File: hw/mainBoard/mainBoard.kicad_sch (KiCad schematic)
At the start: 0 parts

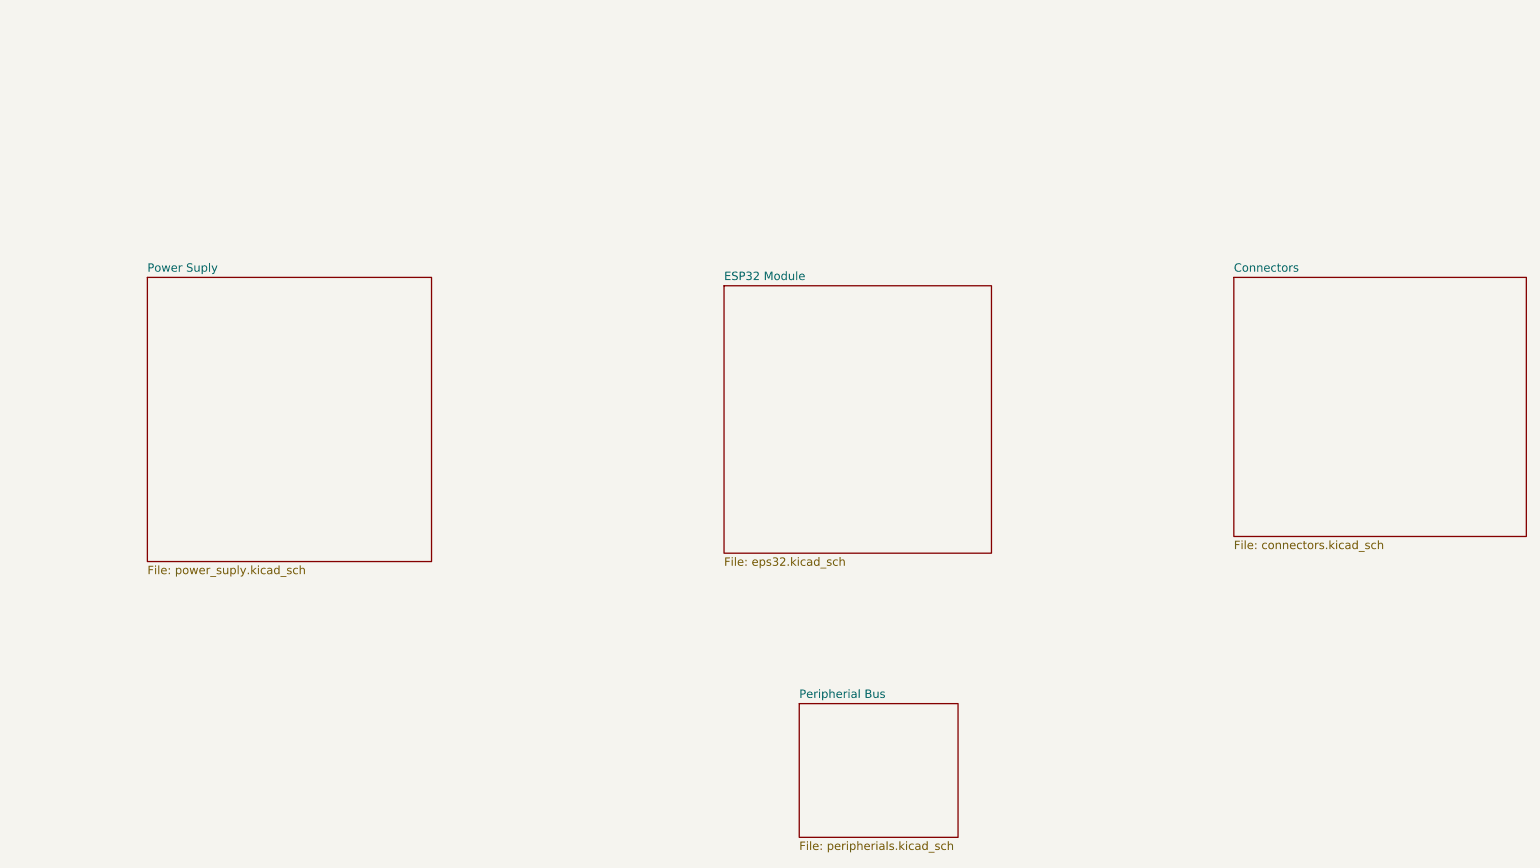
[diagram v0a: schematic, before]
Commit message: hw + blok schema
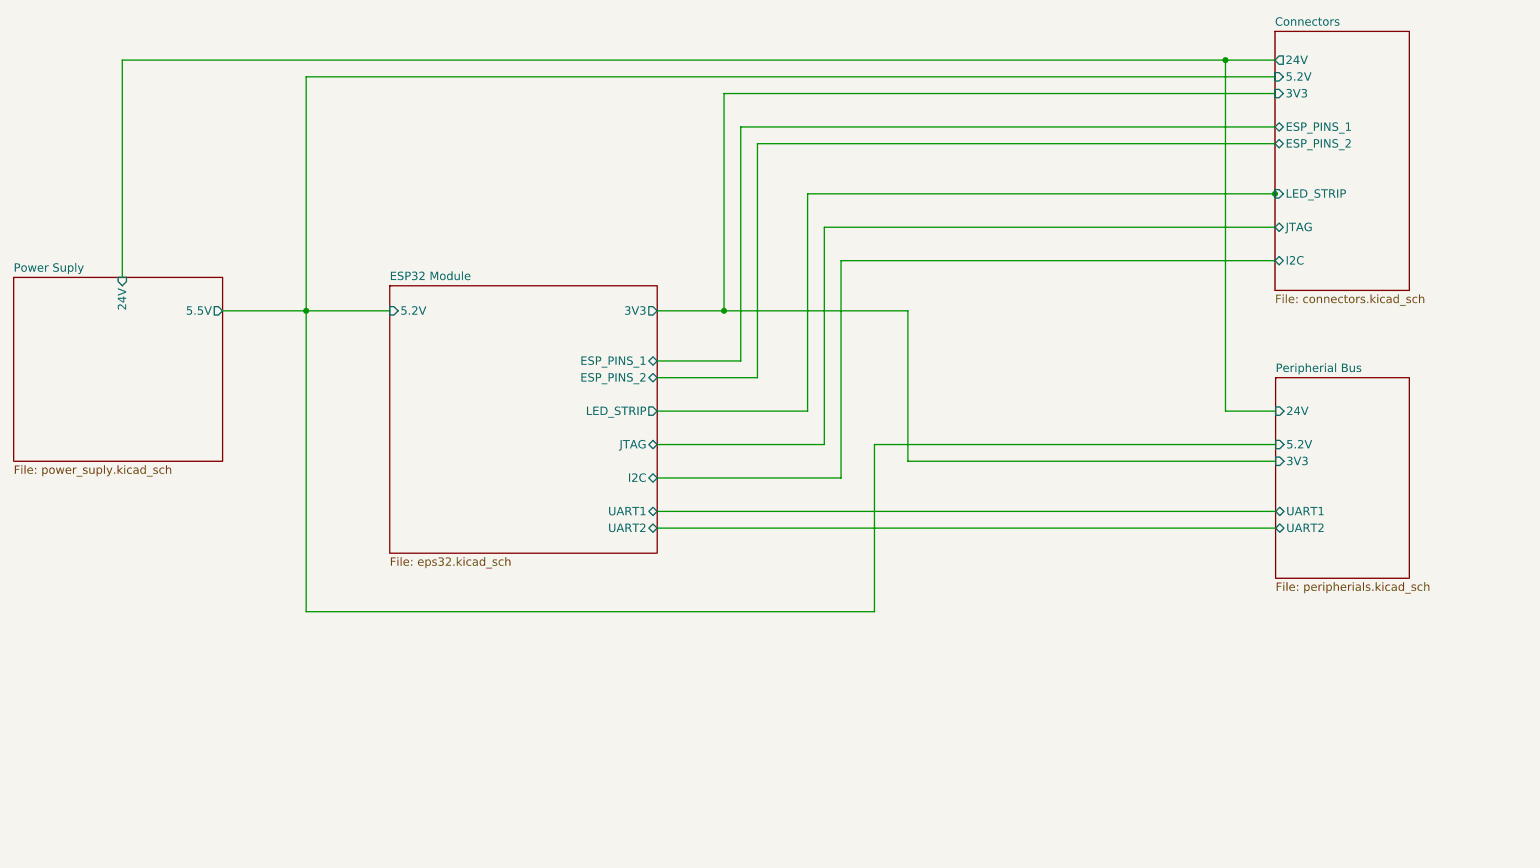
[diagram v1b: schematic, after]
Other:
- sheet Connectors ports: added 24V, 3V3, 5.2V, ESP_PINS_1, ESP_PINS_2, I2C, JTAG, LED_STRIP; removed none
- sheet ESP32 Module ports: added 3V3, 5.2V, ESP_PINS_1, ESP_PINS_2, I2C, JTAG, LED_STRIP, UART1, UART2; removed none
- sheet Peripherial Bus ports: added 24V, 3V3, 5.2V, UART1, UART2; removed none
- sheet Power Suply ports: added 24V, 5.5V; removed none
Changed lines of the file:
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@@
 (kicad_sch (version 20230121) (generator eeschema)
   (paper "A4")
-  (sheet (at 151.13 133.35) (size 24.13 20.32) (fields_autoplaced)
-    (stroke (width 0.1524) (type solid))
-    (fill (color 0 0 0 0.0000))
-    (property "Sheetname" "Peripherial Bus" (at 151.13 132.6384 0)
-      (effects (font (size 1.27 1.27)) (justify left bottom))
-    )
-    (property "Sheetfile" "peripherials.kicad_sch" (at 151.13 154.2546 0)
-      (effects (font (size 1.27 1.27)) (justify left top))
+  (junction (at 215.9 35.56) (diameter 0) (color 0 0 0 0)
+  )
+  (junction (at 139.7 73.66) (diameter 0) (color 0 0 0 0)
+  )
+  (junction (at 223.4202 55.88) (diameter 0) (color 0 0 0 0)
+  )
+  (junction (at 76.2 73.66) (diameter 0) (color 0 0 0 0)
+  )
+  (wire (pts (xy 76.2 119.38) (xy 162.56 119.38))
+    (stroke (width 0) (type default))
+  )
+  (wire (pts (xy 76.2 73.66) (xy 76.2 38.1))
+    (stroke (width 0) (type default))
+  )
+  (wire (pts (xy 152.4 55.88) (xy 223.4202 55.88))
+    (stroke (width 0) (type default))
+  )
+  (wire (pts (xy 129.54 81.28) (xy 142.24 81.28))
+    (stroke (width 0) (type default))
+  )
+  (wire (pts (xy 162.56 93.98) (xy 223.52 93.98))
+    (stroke (width 0) (type default))
+  )
+  (wire (pts (xy 63.5 73.66) (xy 76.2 73.66))
+    (stroke (width 0) (type default))
+  )
+  (wire (pts (xy 139.7 40.64) (xy 223.4202 40.64))
+    (stroke (width 0) (type default))
+  )
+  (wire (pts (xy 76.2 38.1) (xy 223.4202 38.1))
+    (stroke (width 0) (type default))
+  )
+  (wire (pts (xy 129.54 88.9) (xy 152.4 88.9))
+    (stroke (width 0) (type default))
+  )
+  (wire (pts (xy 48.26 35.56) (xy 48.26 68.58))
+    (stroke (width 0) (type default))
+  )
+  (wire (pts (xy 129.54 104.14) (xy 223.52 104.14))
+    (stroke (width 0) (type default))
+  )
+  (wire (pts (xy 167.64 96.52) (xy 223.52 96.52))
+    (stroke (width 0) (type default))
+  )
+  (wire (pts (xy 142.24 45.72) (xy 223.4202 45.72))
+    (stroke (width 0) (type default))
+  )
+  (wire (pts (xy 139.7 73.66) (xy 139.7 40.64))
+    (stroke (width 0) (type default))
+  )
+  (wire (pts (xy 129.54 83.82) (xy 144.78 83.82))
+    (stroke (width 0) (type default))
+  )
+  (wire (pts (xy 162.56 119.38) (xy 162.56 93.98))
+    (stroke (width 0) (type default))
+  )
+  (wire (pts (xy 152.4 88.9) (xy 152.4 55.88))
+    (stroke (width 0) (type default))
+  )
+  (wire (pts (xy 76.2 73.66) (xy 76.2 119.38))
+    (stroke (width 0) (type default))
+  )
+  (wire (pts (xy 157.48 99.06) (xy 157.48 66.04))
+    (stroke (width 0) (type default))
+  )
+  (wire (pts (xy 223.4202 55.88) (xy 223.52 55.88))
+    (stroke (width 0) (type default))
+  )
+  (wire (pts (xy 129.54 99.06) (xy 157.48 99.06))
+    (stroke (width 0) (type default))
+  )
+  (wire (pts (xy 129.54 93.98) (xy 154.94 93.98))
+    (stroke (width 0) (type default))
+  )
+  (wire (pts (xy 142.24 81.28) (xy 142.24 45.72))
+    (stroke (width 0) (type default))
+  )
+  (wire (pts (xy 129.54 73.66) (xy 139.7 73.66))
+    (stroke (width 0) (type default))
+  )
+  (wire (pts (xy 157.48 66.04) (xy 223.4202 66.04))
+    (stroke (width 0) (type default))
+  )
+  (wire (pts (xy 144.78 48.26) (xy 223.4202 48.26))
+    (stroke (width 0) (type default))
+  )
+  (wire (pts (xy 76.2 73.66) (xy 88.9 73.66))
+    (stroke (width 0) (type default))
+  )
+  (wire (pts (xy 215.9 35.56) (xy 48.26 35.56))
+    (stroke (width 0) (type default))
+  )
+  (wire (pts (xy 167.64 73.66) (xy 167.64 96.52))
+    (stroke (width 0) (type default))
+  )
+  (wire (pts (xy 139.7 73.66) (xy 167.64 73.66))
+    (stroke (width 0) (type default))
+  )
+  (wire (pts (xy 223.52 88.9) (xy 215.9 88.9))
+    (stroke (width 0) (type default))
+  )
+  (wire (pts (xy 144.78 83.82) (xy 144.78 48.26))
+    (stroke (width 0) (type default))
+  )
+  (wire (pts (xy 215.9 35.56) (xy 215.9 88.9))
+    (stroke (width 0) (type default))
+  )
+  (wire (pts (xy 154.94 60.96) (xy 223.4202 60.96))
+    (stroke (width 0) (type default))
+  )
+  (wire (pts (xy 129.54 106.68) (xy 223.52 106.68))
+    (stroke (width 0) (type default))
+  )
+  (wire (pts (xy 223.4202 35.56) (xy 215.9 35.56))
+    (stroke (width 0) (type default))
+  )
+  (wire (pts (xy 154.94 93.98) (xy 154.94 60.96))
+    (stroke (width 0) (type default))
+  )
+  (sheet (at 223.52 83.82) (size 20.32 30.48) (fields_autoplaced)
+    (stroke (width 0.1524) (type solid))
+    (fill (color 0 0 0 0.0000))
+    (property "Sheetname" "Peripherial Bus" (at 223.52 83.1084 0)
+      (effects (font (size 1.27 1.27)) (justify left bottom))
+    )
+    (property "Sheetfile" "peripherials.kicad_sch" (at 223.52 114.8846 0)
+      (effects (font (size 1.27 1.27)) (justify left top))
+    )
+    (pin "UART2" bidirectional (at 223.52 106.68 180)
+      (effects (font (size 1.27 1.27)) (justify left))
+    )
+    (pin "UART1" bidirectional (at 223.52 104.14 180)
+      (effects (font (size 1.27 1.27)) (justify left))
+    )
+    (pin "3V3" input (at 223.52 96.52 180)
+      (effects (font (size 1.27 1.27)) (justify left))
+    )
+    (pin "5.2V" input (at 223.52 93.98 180)
+      (effects (font (size 1.27 1.27)) (justify left))
+    )
+    (pin "24V" input (at 223.52 88.9 180)
+      (effects (font (size 1.27 1.27)) (justify left))
     )
     (instances
@@
     )
   )
-  (sheet (at 139.7 69.85) (size 40.64 40.64) (fields_autoplaced)
-    (stroke (width 0.1524) (type solid))
-    (fill (color 0 0 0 0.0000))
-    (property "Sheetname" "ESP32 Module" (at 139.7 69.1384 0)
-      (effects (font (size 1.27 1.27)) (justify left bottom))
-    )
-    (property "Sheetfile" "eps32.kicad_sch" (at 139.7 111.0746 0)
-      (effects (font (size 1.27 1.27)) (justify left top))
+  (sheet (at 88.9 69.85) (size 40.64 40.64) (fields_autoplaced)
+    (stroke (width 0.1524) (type solid))
+    (fill (color 0 0 0 0.0000))
+    (property "Sheetname" "ESP32 Module" (at 88.9 69.1384 0)
+      (effects (font (size 1.27 1.27)) (justify left bottom))
+    )
+    (property "Sheetfile" "eps32.kicad_sch" (at 88.9 111.0746 0)
+      (effects (font (size 1.27 1.27)) (justify left top))
+    )
+    (pin "ESP_PINS_2" bidirectional (at 129.54 83.82 0)
+      (effects (font (size 1.27 1.27)) (justify right))
+    )
+    (pin "ESP_PINS_1" bidirectional (at 129.54 81.28 0)
+      (effects (font (size 1.27 1.27)) (justify right))
+    )
+    (pin "UART1" bidirectional (at 129.54 104.14 0)
+      (effects (font (size 1.27 1.27)) (justify right))
+    )
+    (pin "UART2" bidirectional (at 129.54 106.68 0)
+      (effects (font (size 1.27 1.27)) (justify right))
+    )
+    (pin "JTAG" bidirectional (at 129.54 93.98 0)
+      (effects (font (size 1.27 1.27)) (justify right))
+    )
+    (pin "I2C" bidirectional (at 129.54 99.06 0)
+      (effects (font (size 1.27 1.27)) (justify right))
+    )
+    (pin "3V3" output (at 129.54 73.66 0)
+      (effects (font (size 1.27 1.27)) (justify right))
+    )
+    (pin "5.2V" input (at 88.9 73.66 180)
+      (effects (font (size 1.27 1.27)) (justify left))
+    )
+    (pin "LED_STRIP" output (at 129.54 88.9 0)
+      (effects (font (size 1.27 1.27)) (justify right))
     )
     (instances
@@
     )
   )
-  (sheet (at 52.07 68.58) (size 43.18 43.18) (fields_autoplaced)
-    (stroke (width 0.1524) (type solid))
-    (fill (color 0 0 0 0.0000))
-    (property "Sheetname" "Power Suply" (at 52.07 67.8684 0)
-      (effects (font (size 1.27 1.27)) (justify left bottom))
-    )
-    (property "Sheetfile" "power_suply.kicad_sch" (at 52.07 112.3446 0)
-      (effects (font (size 1.27 1.27)) (justify left top))
+  (sheet (at 31.75 68.58) (size 31.75 27.94) (fields_autoplaced)
+    (stroke (width 0.1524) (type solid))
+    (fill (color 0 0 0 0.0000))
+    (property "Sheetname" "Power Suply" (at 31.75 67.8684 0)
+      (effects (font (size 1.27 1.27)) (justify left bottom))
+    )
+    (property "Sheetfile" "power_suply.kicad_sch" (at 31.75 97.1046 0)
+      (effects (font (size 1.27 1.27)) (justify left top))
+    )
+    (pin "5.5V" output (at 63.5 73.66 0)
+      (effects (font (size 1.27 1.27)) (justify right))
+    )
+    (pin "24V" input (at 48.26 68.58 90)
+      (effects (font (size 1.27 1.27)) (justify right))
     )
     (instances
@@
     )
   )
-  (sheet (at 217.17 68.58) (size 44.45 39.37) (fields_autoplaced)
-    (stroke (width 0.1524) (type solid))
-    (fill (color 0 0 0 0.0000))
-    (property "Sheetname" "Connectors" (at 217.17 67.8684 0)
-      (effects (font (size 1.27 1.27)) (justify left bottom))
-    )
-    (property "Sheetfile" "connectors.kicad_sch" (at 217.17 108.5346 0)
-      (effects (font (size 1.27 1.27)) (justify left top))
-    )
-    (instances
+  (sheet (at 223.4202 31.1944) (size 20.4198 39.37) (fields_autoplaced)
+    (stroke (width 0.1524) (type solid))
+    (fill (color 0 0 0 0.0000))
+    (property "Sheetname" "Connectors" (at 223.4202 30.4828 0)
+      (effects (font (size 1.27 1.27)) (justify left bottom))
+    )
+    (property "Sheetfile" "connectors.kicad_sch" (at 223.4202 71.149 0)
+      (effects (font (size 1.27 1.27)) (justify left top))
+    )
+    (pin "JTAG" bidirectional (at 223.4202 60.96 180)
+      (effects (font (size 1.27 1.27)) (justify left))
+    )
+    (pin "ESP_PINS_2" bidirectional (at 223.4202 48.26 180)
+      (effects (font (size 1.27 1.27)) (justify left))
+    )
+    (pin "ESP_PINS_1" bidirectional (at 223.4202 45.72 180)
+      (effects (font (size 1.27 1.27)) (justify left))
+    )
+    (pin "I2C" bidirectional (at 223.4202 66.04 180)
+      (effects (font (size 1.27 1.27)) (justify left))
+    )
+    (pin "3V3" input (at 223.4202 40.64 180)
+      (effects (font (size 1.27 1.27)) (justify left))
+    )
+    (pin "24V" output (at 223.4202 35.56 180)
+      (effects (font (size 1.27 1.27)) (justify left))
+    )
+    (pin "LED_STRIP" input (at 223.4202 55.88 180)
+      (effects (font (size 1.27 1.27)) (justify left))
+    )
+    (pin "5.2V" input (at 223.4202 38.1 180)
+      (effects (font (size 1.27 1.27)) (justify left))
+    )
+    (instances
